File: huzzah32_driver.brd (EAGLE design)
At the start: 100 x 80 mm, 9 parts, among them IC1 7805T, J1 1X2-3.5MM, X1 C-GRID-16-70543, X2 C-GRID-12-70543, X3 22-23-2021, X4 22-23-2021

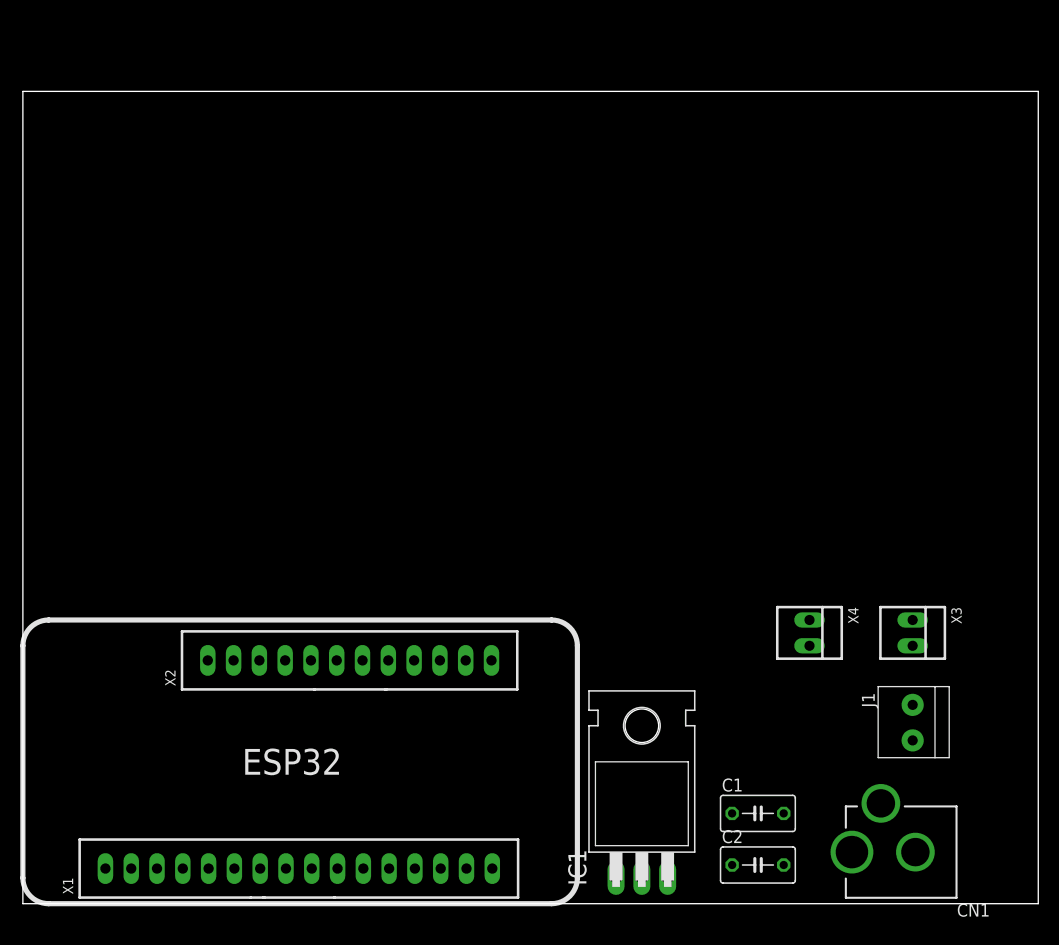
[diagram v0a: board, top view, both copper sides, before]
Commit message: I've been working on this for like 6 hours and now it's 4am you expect me to write a commit message? -finished the board
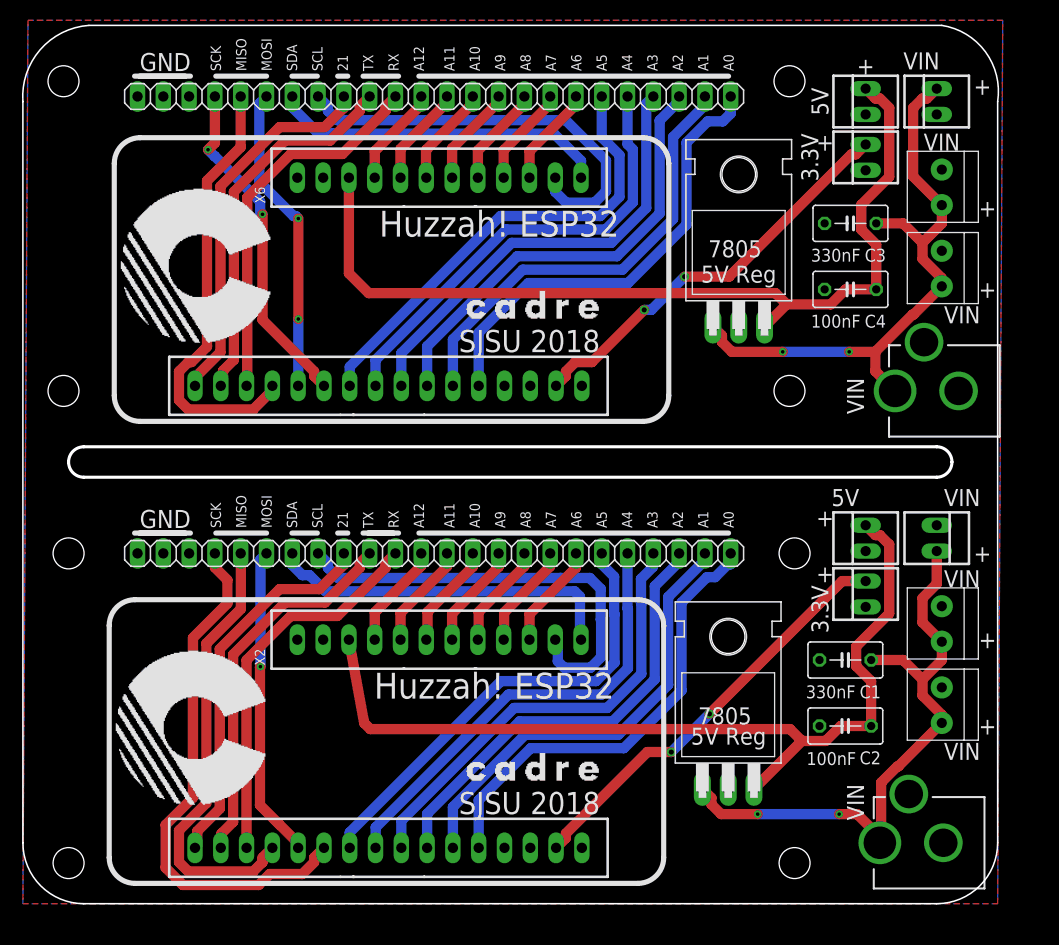
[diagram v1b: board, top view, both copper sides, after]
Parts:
- added C3: 330nF, resistor:C050-035X075
- added C4: 100nF, resistor:C050-035X075
- added CN2: (no value), adafruit:DCJACK_2MM_PTH
- added IC2: 7805T, linear:TO220H
- added J2, J3, J4: 1X2-3.5MM, adafruit:1X2-3.5MM
- added JP1, JP2: (no value), pinhead:1X24
- added X10, X7, X8, X9: 22-23-2021, con-molex:22-23-2021
- added X5: C-GRID-16-70543, lumiled_boards:70543-16
- added X6: C-GRID-12-70543, lumiled_boards:70543-12
- moved C1 17.4 mm to (81.0, 24.0), turned to 180 degrees
- moved C2 16.2 mm to (81.0, 17.5), turned to 180 degrees
- moved IC1 12.2 mm to (69.5, 21.5)
- moved X4 10.8 mm to (83.0, 36.0), turned to 90 degrees
- moved X3 9.63 mm to (90.0, 36.0)
- moved X1 9.05 mm to (36.0, 5.50)
- moved X2 9.05 mm to (41.0, 26.0)
- moved J1 3.35 mm to (90.5, 19.5)
- moved CN1 2.90 mm to (98.0, 6.00)
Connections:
- removed net A0_DAC2: X1.12
- removed net A1_DAC1: X1.11
- removed net A2_I34: X1.10
- removed net A3_I39: X1.9
- removed net A4_IO36: X1.8
- removed net A5_IO4: X1.7
- removed net EN: X2.2
- removed net IO12_A11: X2.5
- removed net IO13_A12: X2.4
- removed net IO14_A6: X2.10
- removed net IO15_A8: X2.8
- removed net IO16: X1.3
- removed net IO17: X1.2
- removed net IO21: X1.1
- removed net IO27_A10: X2.6
- removed net IO32_A7: X2.9
- removed net IO33_A9: X2.7
- removed net MISO: X1.4
- removed net MOSI: X1.5
- removed net N$26: X1.14
- removed net RESET: X1.16
- removed net SCK: X1.6
- removed net SCL: X2.11
- removed net SDA: X2.12
- removed net VBAT: X2.1
- new net A0_DAC2_B1: JP1.1, X1.12
- new net A0_DAC2_B2: JP2.1, X5.12
- new net A1_DAC1_B1: JP1.2, X1.11
- new net A1_DAC1_B2: JP2.2, X5.11
- new net A2_I34_B1: JP1.3, X1.10
- new net A2_I34_B2: JP2.3, X5.10
- new net A3_I39_B1: JP1.4, X1.9
- new net A3_I39_B2: JP2.4, X5.9
- new net A4_IO36_B1: JP1.5, X1.8
- new net A4_IO36_B2: JP2.5, X5.8
- new net A5_IO4_B1: JP1.6, X1.7
- new net A5_IO4_B2: JP2.6, X5.7
- new net IO12_A11_B1: JP1.12, X2.5
- new net IO12_A11_B2: JP2.12, X6.5
- new net IO13_A12_B1: JP1.13, X2.4
- new net IO13_A12_B2: JP2.13, X6.4
- new net IO14_A6_B1: JP1.7, X2.10
- new net IO14_A6_B2: JP2.7, X6.10
- new net IO15_A8_B1: JP1.9, X2.8
- new net IO15_A8_B2: JP2.9, X6.8
- new net IO16_B1: JP1.14, X1.3
- new net IO16_B2: JP2.14, X5.3
- new net IO17_B1: JP1.15, X1.2
- new net IO17_B2: JP2.15, X5.2
- new net IO21_B1: JP1.16, X1.1
- new net IO21_B2: JP2.16, X5.1
- new net IO27_A10_B1: JP1.11, X2.6
- new net IO27_A10_B2: JP2.11, X6.6
- new net IO32_A7_B1: JP1.8, X2.9
- new net IO32_A7_B2: JP2.8, X6.9
- new net IO33_A9_B1: JP1.10, X2.7
- new net IO33_A9_B2: JP2.10, X6.7
- new net MISO_B1: JP1.20, X1.4
- new net MISO_B2: JP2.20, X5.4
- new net MOSI_B1: JP1.19, X1.5
- new net MOSI_B2: JP2.19, X5.5
- new net SCK_B1: JP1.21, X1.6
- new net SCK_B2: JP2.21, X5.6
- new net SCL_B1: JP1.17, X2.11
- new net SCL_B2: JP2.17, X6.11
- new net SDA_B1: JP1.18, X2.12
- new net SDA_B2: JP2.18, X6.12
- net +3V3: now also X10.2, X5.15, X9.2
- net +5V: now also C4.1, IC2.3, X6.3, X8.2
- net GND: now also C3.2, C4.2, CN2.GND, CN2.GNDBREAK, IC2.2, J2.1, J3.1, J4.1, JP1.22, JP1.23, JP1.24, JP2.22, JP2.23, JP2.24, X10.1, X5.13, X7.1, X8.1, X9.1
- net V+: now also C3.1, CN2.PWR, IC2.1, J2.2, J3.2, J4.2, X7.2
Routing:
- net +5V: track 0.00 -> 178.3 mm
- net V+: track 0.00 -> 120.1 mm, vias 0 -> 4
- net +3V3: track 0.00 -> 82.2 mm, vias 0 -> 4
- net SCK_B1: track 0.00 -> 52.1 mm
- net A5_IO4_B2: track 0.00 -> 46.0 mm
- net A5_IO4_B1: track 0.00 -> 45.8 mm
- net A0_DAC2_B2: track 0.00 -> 45.4 mm
- net A0_DAC2_B1: track 0.00 -> 45.3 mm
- net A4_IO36_B2: track 0.00 -> 45.0 mm
- net A4_IO36_B1: track 0.00 -> 44.7 mm
- net A3_I39_B1: track 0.00 -> 44.7 mm
- net A1_DAC1_B1: track 0.00 -> 44.7 mm
- net A2_I34_B1: track 0.00 -> 44.7 mm
- net A1_DAC1_B2: track 0.00 -> 44.5 mm
- net A3_I39_B2: track 0.00 -> 44.5 mm
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- added copper zone on layer 1, net GND
- added copper zone on layer 16, net GND
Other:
- board size 100 x 80 mm -> 96.1 x 86.5 mm
- board text added: "+"
- board text added: "12"
- board text added: "13"
- board text added: "14"
- board text added: "15"
- board text added: "16"
- board text added: "17"
- board text added: "18"
- board text added: "19"
- board text added: "21"
- board text added: "21: Digital Only"
- board text added: "22"
- board text added: "23"
- board text added: "27"
- board text added: "3.3V"
- board text added: "32"
- board text added: "33"
- board text added: "34"
- board text added: "36"
- board text added: "39"
- board text added: "4"
- board text added: "5"
- board text added: "5V"
- board text added: "5V Reg"
- board text added: "7805"
- board text added: "A0"
- board text added: "A0-A12: Analog Pins"
- board text added: "A1"
- board text added: "A10"
- board text added: "A11"
- board text added: "A12"
- board text added: "A2"
- board text added: "A3"
- board text added: "A4"
- board text added: "A5"
- board text added: "A6"
- board text added: "A7"
- board text added: "A8"
- board text added: "A9"
- board text added: "DAC1"
- board text added: "DAC1, DAC2: Digital to Analog Pins"
- board text added: "DAC2"
- board text added: "GND"
- board text added: "Huzzah! ESP32"
- board text added: "I2C: SCL, SDA"
- board text added: "MISO"
- board text added: "MOSI"
- board text added: "Pin Descriptions"
- board text added: "RX"
- board text added: "RX, TX: Serial Data"
- board text added: "SCK"
- board text added: "SCL"
- board text added: "SDA"
- board text added: "SJSU 2018"
- board text added: "SPI: MOSI, MISO, SCK"
- board text added: "TX"
- board text added: "VIN"
- board text removed: "ESP32"
